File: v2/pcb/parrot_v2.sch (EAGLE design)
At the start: 45 parts, among them Q1 PNO8L07, Q2 PNO8L07, Q3 PNO8L07, Q4 PNO8L07, U1 SHTC3

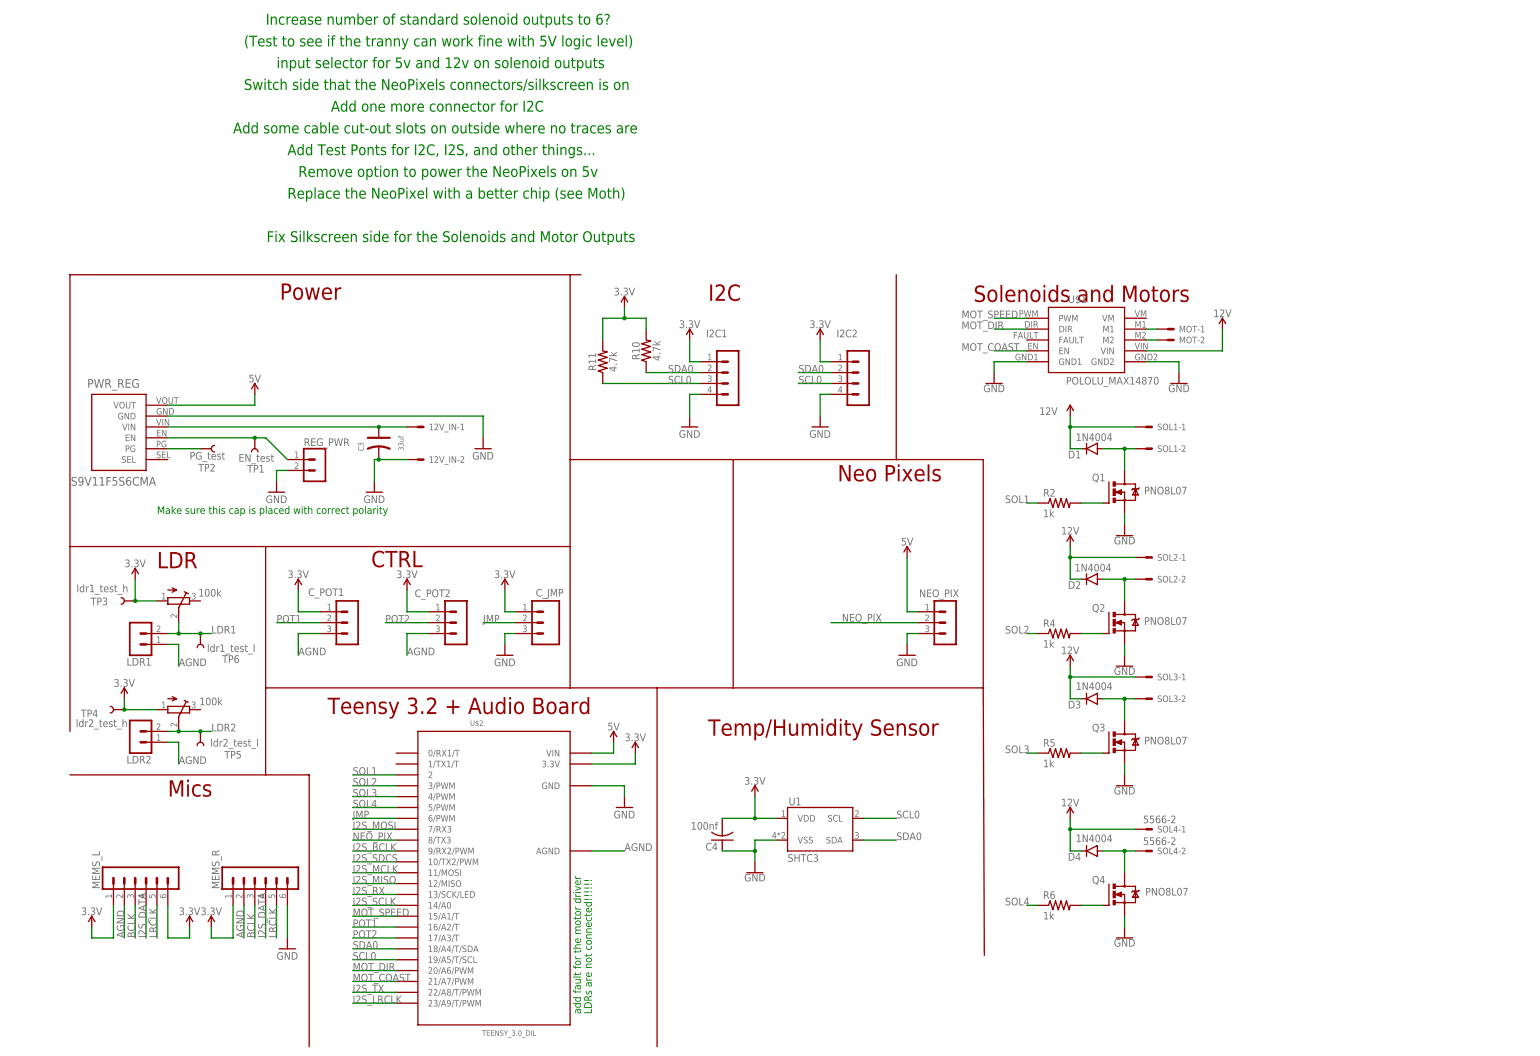
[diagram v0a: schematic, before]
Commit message: moving along, added pdf, jpg, and png to git lfs
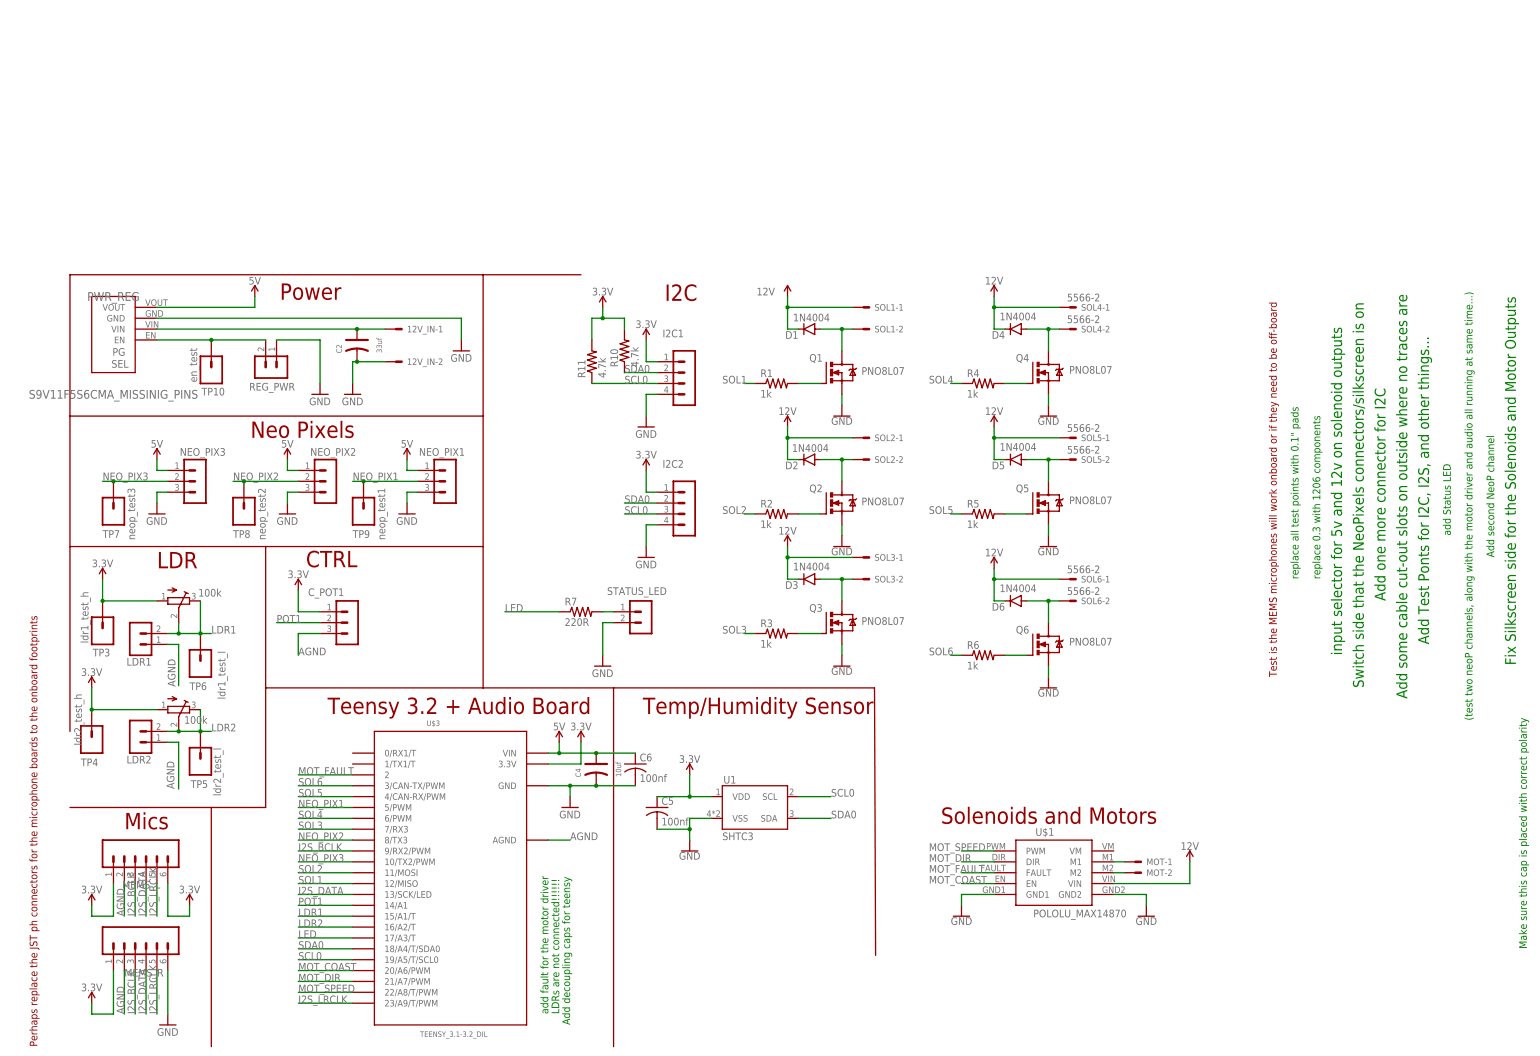
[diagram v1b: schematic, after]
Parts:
- removed C3: 33uf, Seeed-Capacitor:DIP-ALUMINUM-47UF-16V(D5-H7MM)
- removed C_JMP: (no value), SparkFun-Connectors:CONN_03
- removed C_POT2, NEO_PIX: B3B-PH-K, con-jst-ph:B3B-PH-K
- removed TP1: EN_test, SparkFun-Connectors:TEST-POINTTP_15TH_THRU
- removed TP2: PG_test, SparkFun-Connectors:TEST-POINTTP_15TH_THRU
- removed U$2: TEENSY_3.0_DIL, teensy_3_and_LC:TEENSY_3.0_DIL
- added C2: 33uf, Seeed-Capacitor:DIP-ALUMINUM-47UF-16V(D5-H7MM)
- added C5, C6: 100nf, adafruit:C-USC2012
- added D5, D6: 1N4004, SparkFun-DiscreteSemi:DIODEPTH
- added NEO_PIX1, NEO_PIX2, NEO_PIX3: B3B-PH-K, con-jst-ph:B3B-PH-K
- added Q5, Q6: PNO8L07, transistor-power:IRF540
- added R1, R3: 1k, adafruit:R-US_M1206
- added R7: 220R, adafruit:R-US_M1206
- added SOL5, SOL6: 5566-2, con-molex:5566-2
- added STATUS_LED: B2B-PH-K, con-jst-ph:B2B-PH-K
- added TP10: en_test, SparkFun-Connectors:CONN_01
- added TP7: neop_test3, SparkFun-Connectors:CONN_01
- added TP8: neop_test2, SparkFun-Connectors:CONN_01
- added TP9: neop_test1, SparkFun-Connectors:CONN_01
- added U$3: TEENSY_3.1-3.2_DIL, teensy_3_and_LC:TEENSY_3.1-3.2_DIL
- C4: value 100nf -> 10uf; device adafruit:C-USC2012 -> Seeed-Capacitor:DIP-ALUMINUM-47UF-16V(D5-H7MM)
- MEMS_L, MEMS_R: value B6B-PH-K -> (none); device con-jst-ph:B6B-PH-K -> SparkFun-Connectors:CONN_06POLAR
- PWR_REG: value S9V11F5S6CMA -> S9V11F5S6CMA_MISSINIG_PINS; device nathans-custom-parts:S9V11F5S6CMA -> nathans-custom-parts:S9V11F5S6CMA_MISSINIG_PINS
- R10, R11: device SparkFun-Resistors:10OHM-HORIZ-1/4W-1% -> adafruit:R-US_M1206
- R2, R4, R5, R6: device SparkFun-Resistors:10KOHM-HORIZ-1/4W-5% -> adafruit:R-US_M1206
- TP3, TP4, TP5, TP6: device SparkFun-Connectors:TEST-POINTTP_15TH_THRU -> SparkFun-Connectors:CONN_01
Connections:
- removed net BCLK: MEMS_L.3, MEMS_R.3
- removed net I2S_MCLK: U$2.11/MOSI
- removed net I2S_MISO: U$2.12/MISO
- removed net I2S_MOSI: U$2.7/RX3
- removed net I2S_RX: U$2.13/SCK/LED
- removed net I2S_SCLK: U$2.14/A0
- removed net I2S_SDCS: U$2.10/TX2/PWM
- removed net I2S_TX: U$2.22/A8/T/PWM
- removed net JMP: C_JMP.2, U$2.6/PWM
- removed net LRCLK: MEMS_L.5, MEMS_R.5
- removed net N$15: U$1.GND1
- removed net N$3: PWR_REG.PG, TP2.1
- removed net NEO_PIX: NEO_PIX.2, U$2.8/TX3
- removed net POT2: C_POT2.2, U$2.17/A3/T
- new net LED: R7.1, U$3.17/A3/T
- new net MOT_FAULT: U$1.FAULT, U$3.2
- new net N$1: Q5.G, R5.2
- new net N$2: D5.A, Q5.D, SOL5-2.S
- new net N$4: Q6.G, R6.2
- new net N$6: D6.A, Q6.D, SOL6-2.S
- new net N$7: R7.2, STATUS_LED.1
- new net NEO_PIX1: NEO_PIX1.2, TP9.1, U$3.5/PWM
- new net NEO_PIX2: NEO_PIX2.2, TP8.1, U$3.8/TX3
- new net NEO_PIX3: NEO_PIX3.2, TP7.1, U$3.10/TX2/PWM
- new net SOL5: R5.1, U$3.4/CAN-RX/PWM
- new net SOL6: R6.1, U$3.3/CAN-TX/PWM
- net 12V: now also C2.+, D5.C, D6.C, SOL5-1.S, SOL6-1.S; no longer C3.+
- net 3.3V: now also C5.1, U$3.3.3V; no longer C4.2, C_JMP.1, C_POT2.1, U$2.3.3V
- net 5V: now also C4.+, C6.1, NEO_PIX1.1, NEO_PIX2.1, NEO_PIX3.1, U$3.VIN; no longer NEO_PIX.1, U$2.VIN
- net AGND: now also U$3.AGND; no longer C_POT2.3, U$2.AGND
- net GND: now also C2.-, C4.-, C5.2, C6.2, NEO_PIX1.3, NEO_PIX2.3, NEO_PIX3.3, Q5.S, Q6.S, REG_PWR.1, STATUS_LED.2, U$1.GND1, U$3.GND; no longer C3.-, C4.1, C_JMP.3, NEO_PIX.3, REG_PWR.2, U$2.GND
- net I2S_BCLK: now also MEMS_L.3, MEMS_R.3, U$3.9/RX2/PWM; no longer U$2.9/RX2/PWM
- net I2S_DATA: now also U$3.13/SCK/LED
- net I2S_LRCLK: now also MEMS_L.5, MEMS_R.5, U$3.23/A9/T/PWM; no longer U$2.23/A9/T/PWM
- net LDR1: now also TM1.E, U$3.15/A1/T
- net LDR2: now also TM2.E, U$3.16/A2/T
- net MOT_COAST: now also U$3.20/A6/PWM; no longer U$2.21/A7/PWM
- net MOT_DIR: now also U$3.21/A7/PWM; no longer U$2.20/A6/PWM
- net MOT_SPEED: now also U$3.22/A8/T/PWM; no longer U$2.15/A1/T
- net N$10: now also REG_PWR.2, TP10.1; no longer REG_PWR.1, TP1.1
- net N$11: now also R3.2; no longer R5.2
- net N$13: now also R4.2; no longer R6.2
- net N$24: now also R1.2; no longer R2.2
- net N$5: now also R2.2; no longer R4.2
- net POT1: now also U$3.14/A1; no longer U$2.16/A2/T
- net SCL0: now also U$3.19/A5/T/SCL0; no longer U$2.19/A5/T/SCL
- net SDA0: now also U$3.18/A4/T/SDA0; no longer U$2.18/A4/T/SDA
- net SOL1: now also R1.1, U$3.12/MISO; no longer R2.1, U$2.2
- net SOL2: now also R2.1, U$3.11/MOSI; no longer R4.1, U$2.3/PWM
- net SOL3: now also R3.1, U$3.7/RX3; no longer R5.1, U$2.4/PWM
- net SOL4: now also R4.1, U$3.6/PWM; no longer R6.1, U$2.5/PWM
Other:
- note added: "(test two neoP channels, along with the motor driver and audio all running at same time...)"
- note added: "Add decoupling caps for teensy"
- note added: "Add second NeoP channel"
- note added: "Perhaps replace the JST ph connectors for the microphone boards to the onboard footprints"
- note added: "Test is the MEMS microphones will work onboard or if they need to be off-board"
- note added: "add Status LED"
- note added: "replace 0.3 with 1206 components"
- note added: "replace all test points with 0.1" pads"
- note removed: "(Test to see if the tranny can work fine with 5V logic level)"
- note removed: "Increase number of standard solenoid outputs to 6?"
- note removed: "Remove option to power the NeoPixels on 5v"
- note removed: "Replace the NeoPixel with a better chip (see Moth)"
- moved on the sheet: 12V_IN-1, 12V_IN-2, D1, D2, D3, D4, I2C1, I2C2, MEMS_L, MEMS_R, MOT-1, MOT-2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
